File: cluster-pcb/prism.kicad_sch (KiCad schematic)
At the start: 5 parts, among them J501 Conn_01x04_P3.5mm_TBH_Horizon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, U501 MAX13431E

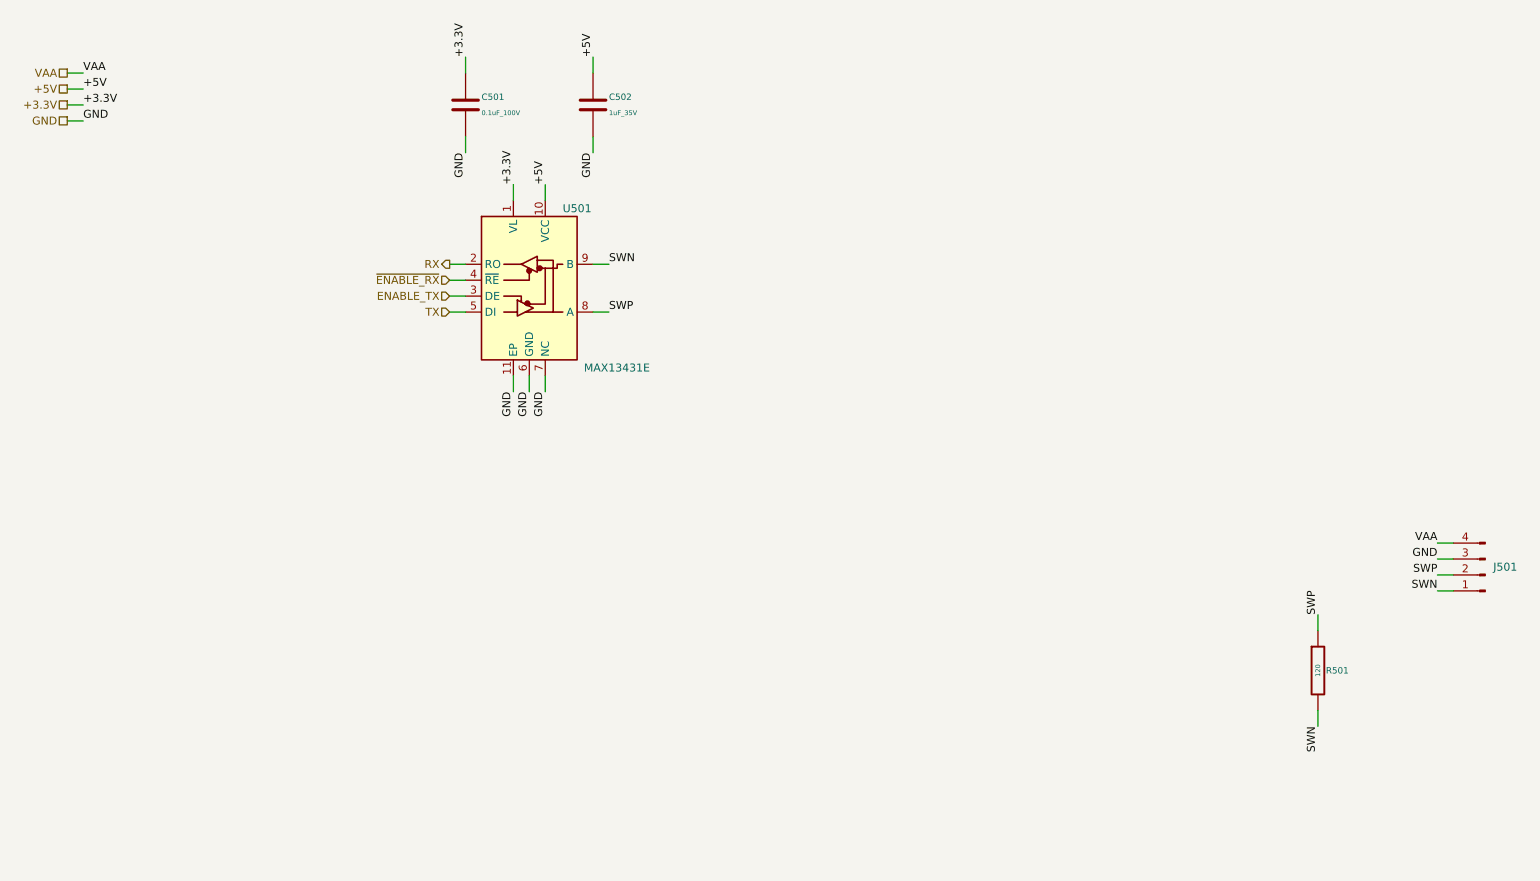
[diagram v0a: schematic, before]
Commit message: Update schematic
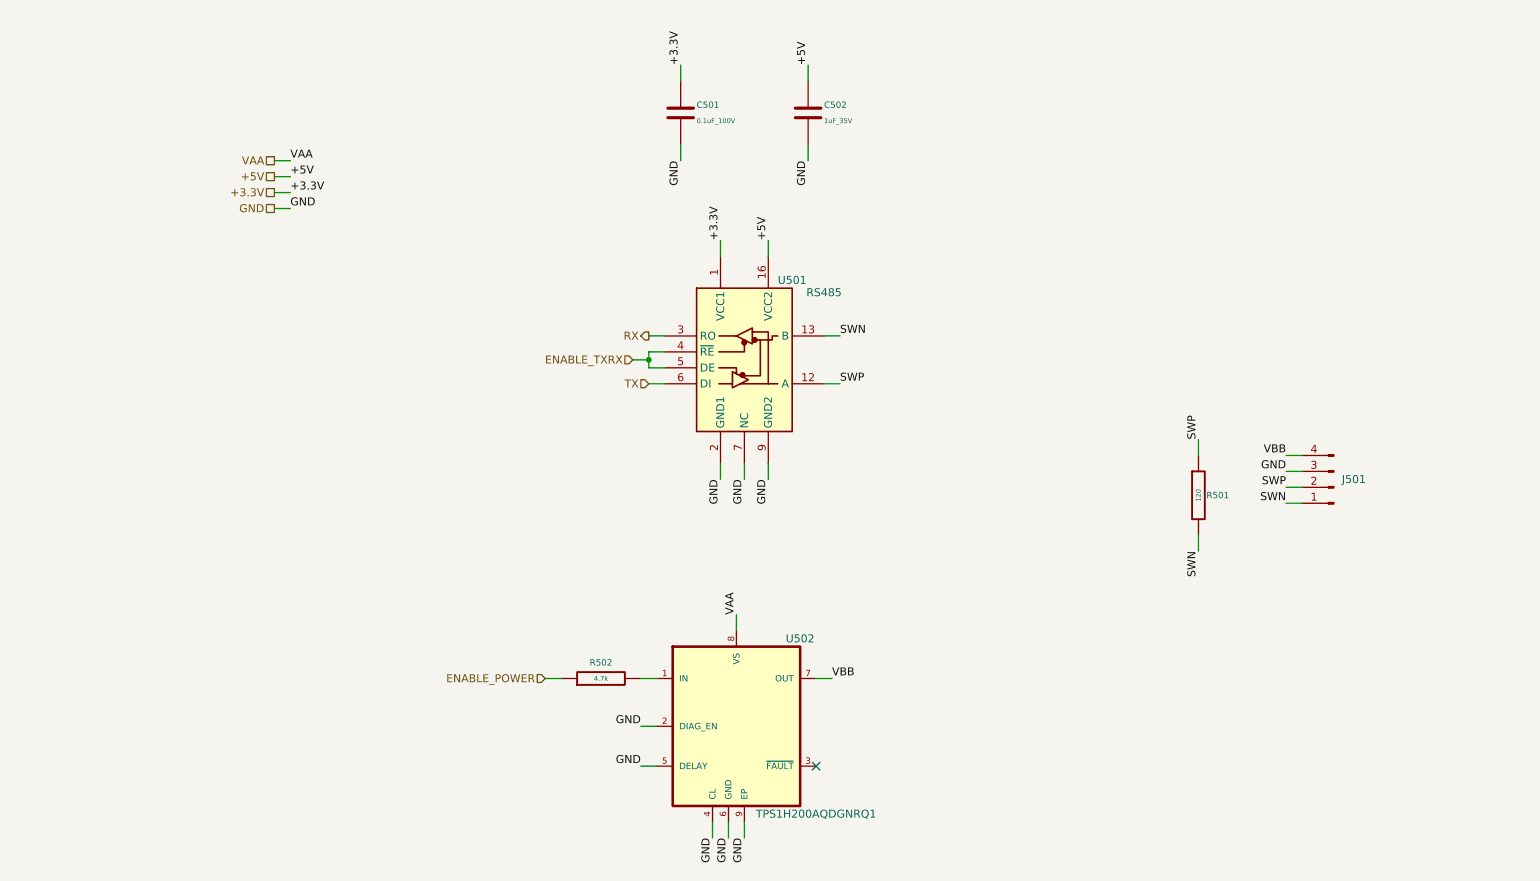
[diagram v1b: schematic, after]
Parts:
- removed U501: MAX13431E, Janelia:21-0137I_T1033-1_MXM, symbol Janelia:MAX13431E
- added R502: 4.7k, Janelia:R_0402_1005Metric, symbol Janelia:R_4.7k_0402
- added U501: RS485, Janelia:DW0016B, symbol Janelia:Interface_RS485_ISO1410
- added U502: TPS1H200AQDGNRQ1, Janelia:SOP65P490X110-9N, symbol Janelia:TPS1H200AQDGNRQ1
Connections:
- net +3.3V: now also U501.1 (VCC1)
- net +5V: now also U501.16 (VCC2)
- net RX: now also U501.3 (RO)
- net SWN: now also U501.13 (B)
- net SWP: now also U501.12 (A)
- net TX: now also U501.6 (DI)
- net VAA: now also U502.8 (VS); no longer J501.4 (Pin_4)
- net GND renamed GND1
- net GND1: now also U501.10 (NC), U501.11 (NC), U501.14 (NC), U501.15 (GND2), U501.2 (GND1), U501.7 (NC), U501.8 (GND1), U501.9 (GND2), U502.2 (DIAG_EN), U502.4 (CL), U502.5 (DELAY), U502.6 (GND), U502.9 (EP)
- new net: R502.2, U502.1 (IN)
- new net ENABLE_POWER: R502.1
- new net ENABLE_TXRX: U501.4 (~{RE}), U501.5 (DE)
- new net VBB: J501.4 (Pin_4), U502.7 (OUT)
- no-connect marks 0 -> 1
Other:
- moved on the sheet: C501, C502, J501, R501
